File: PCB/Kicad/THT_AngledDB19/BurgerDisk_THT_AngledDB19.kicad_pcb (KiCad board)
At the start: 2 copper layers, 93.7 x 73.4 mm, 18 parts, among them J1 Daisy port in, J2 MicroSD module, J3 UART, J4 Daisy port out, U1 PC817

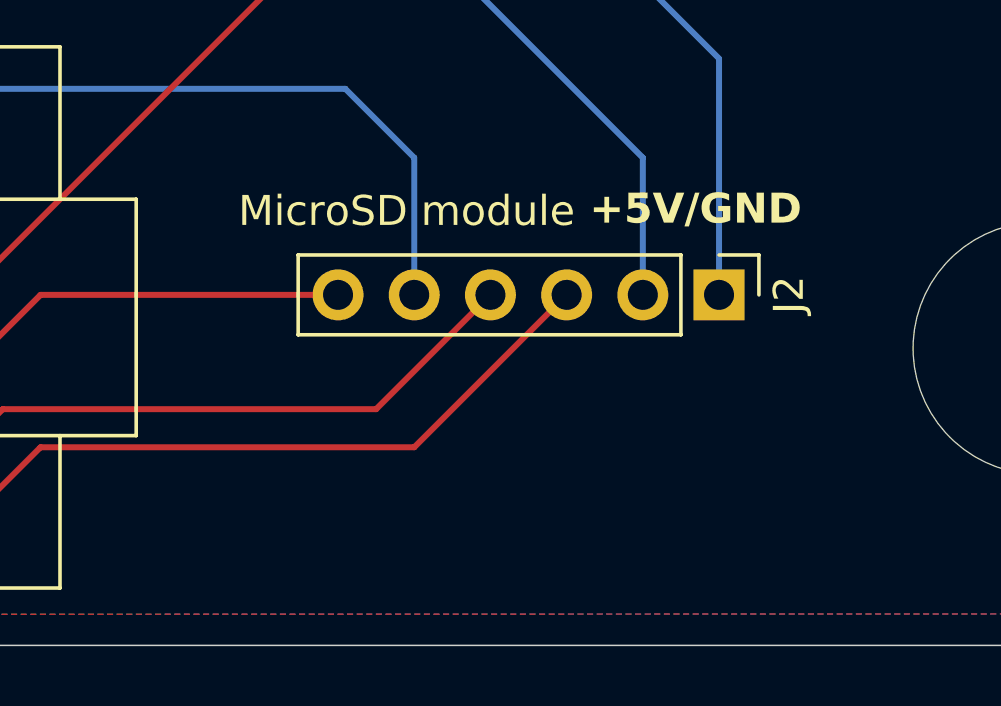
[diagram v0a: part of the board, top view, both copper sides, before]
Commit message: Small esthetic fixes
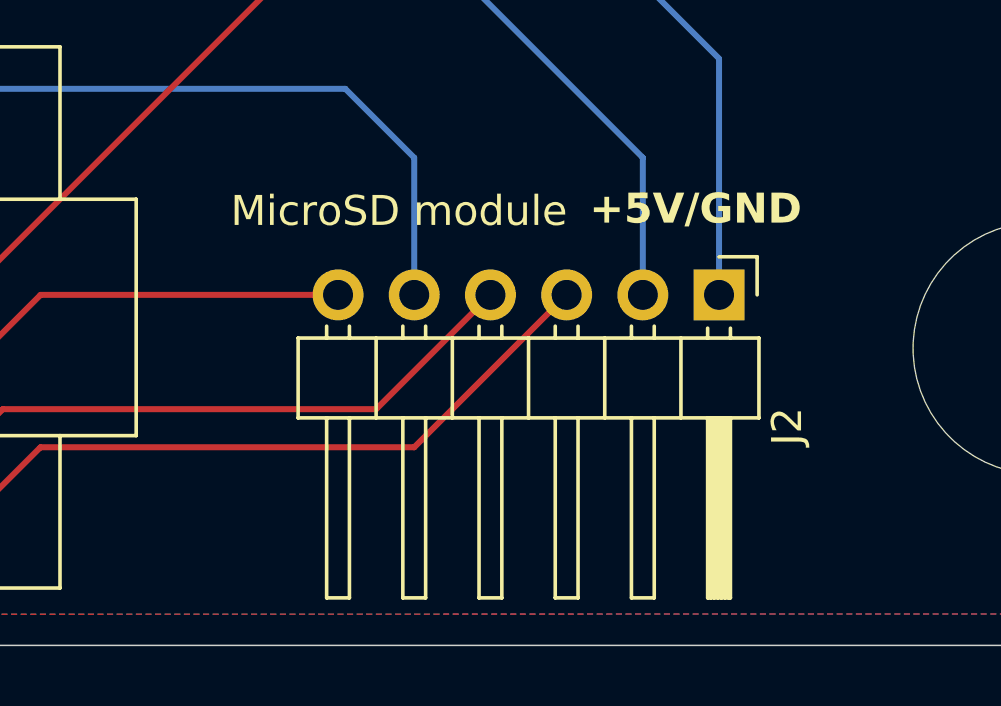
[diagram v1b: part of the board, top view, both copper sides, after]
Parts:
- J2: footprint Connector_PinHeader_2.54mm:PinHeader_1x06_P2.54mm_Vertical -> Connector_PinHeader_2.54mm:PinHeader_1x06_P2.54mm_Horizontal
